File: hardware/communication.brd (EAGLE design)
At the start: 33.5 x 34.6 mm, 39 parts, among them J1 MICRO_USB_B_HIROSE_ZX62-B-5PA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, U2 NJM12888F, X1 FA-238

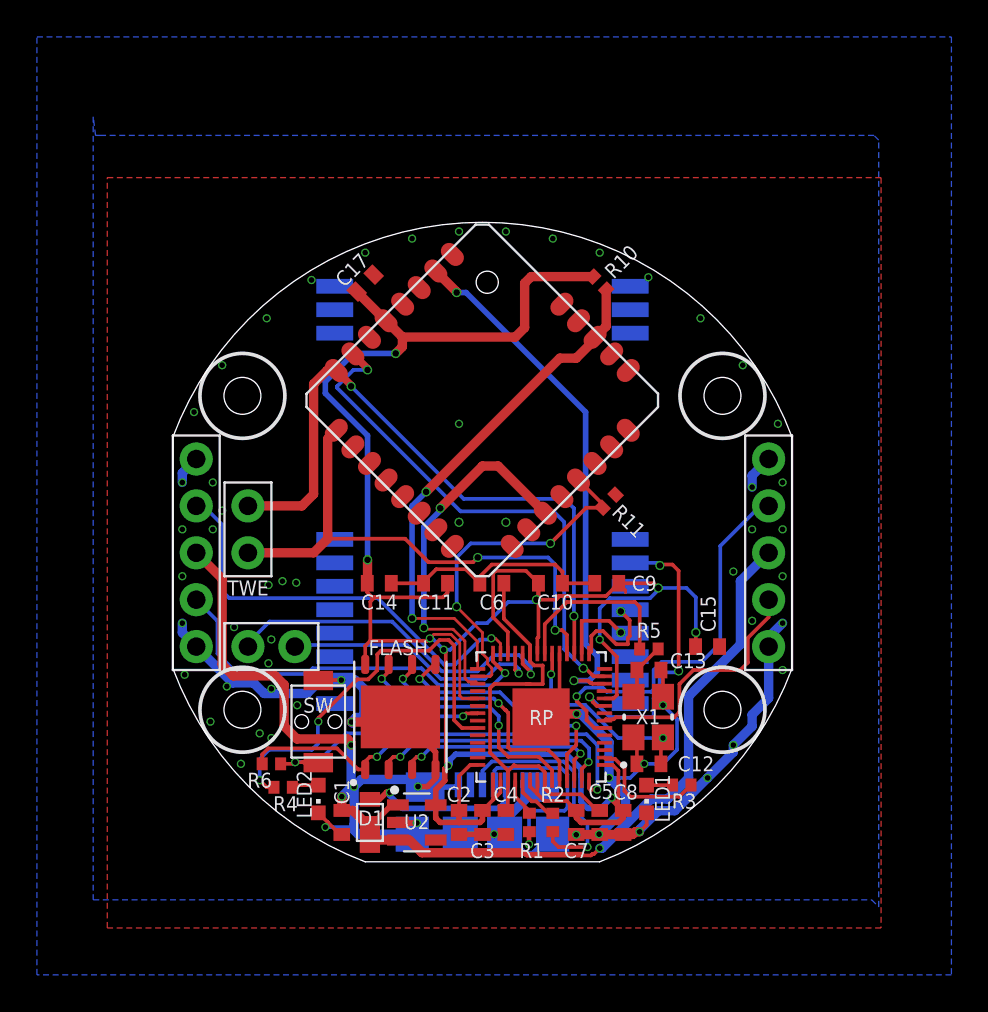
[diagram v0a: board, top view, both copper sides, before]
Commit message: communication_修正
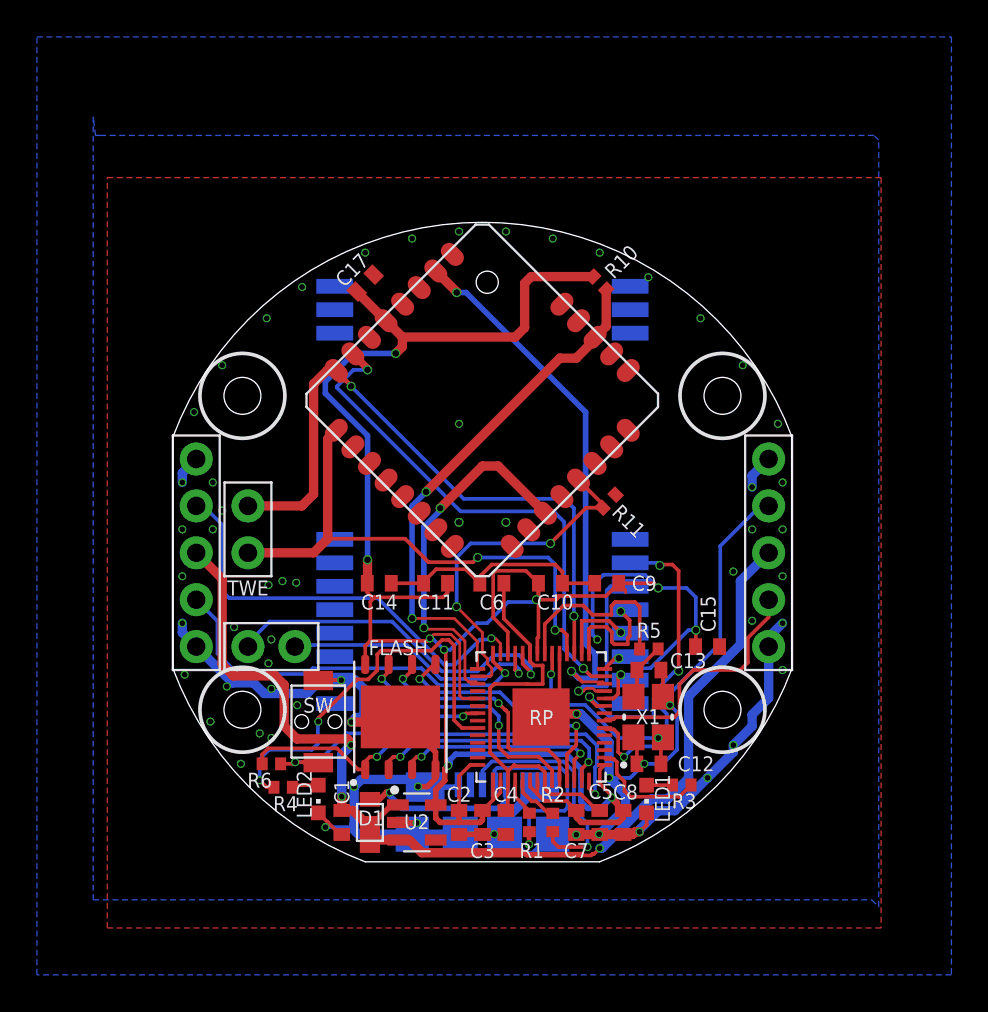
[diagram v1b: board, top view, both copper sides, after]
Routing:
- net LORA_M1: track 0.00 -> 9.72 mm, vias 0 -> 1
- net VDD: track 137.3 -> 142.1 mm, vias 10 -> 11
- net LORA_AUX: track 0.00 -> 1.67 mm, vias 0 -> 1
- net LORA_TRX: track 5.39 -> 6.74 mm
- net TWE_RTX: track 35.8 -> 36.5 mm
- net TX1: track 21.2 -> 20.5 mm
- net XOUT1: track 9.62 -> 10.3 mm
- net TWE_PGM: track 28.8 -> 29.4 mm
- net LORA_RTX: track 4.15 -> 4.67 mm

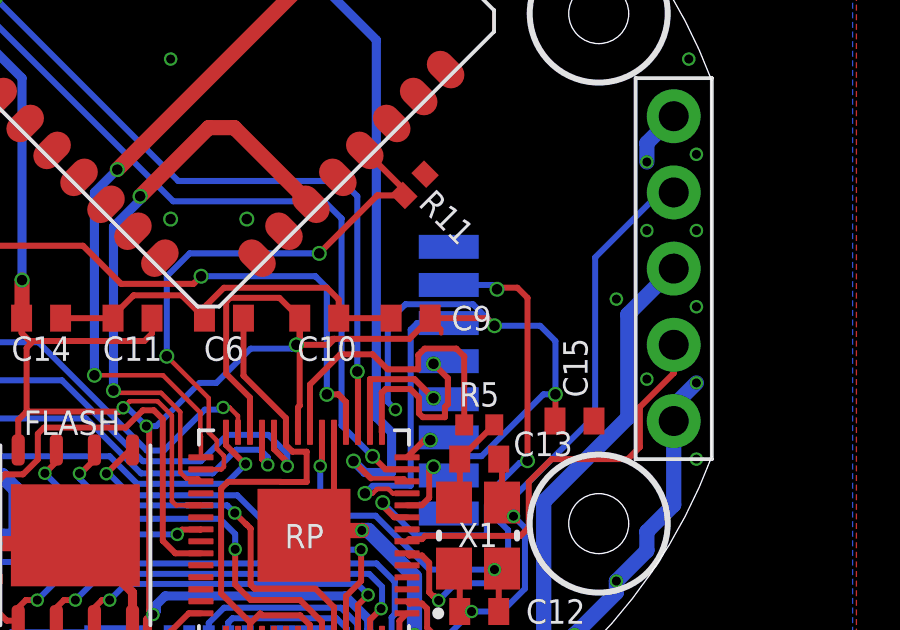
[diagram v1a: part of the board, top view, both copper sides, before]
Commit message: 回路微修正
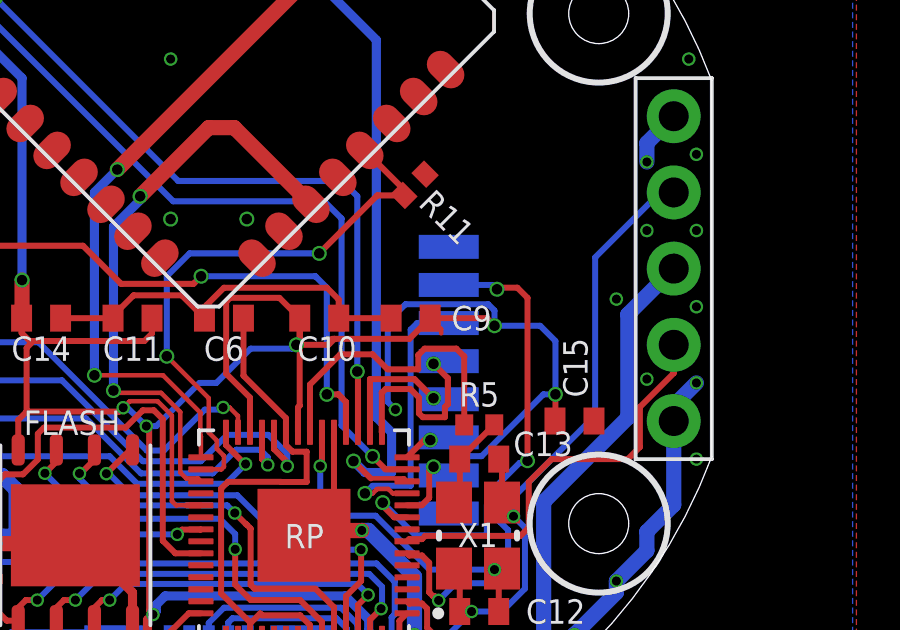
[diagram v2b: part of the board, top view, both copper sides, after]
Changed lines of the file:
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@@
 <param name="mdViaVia" value="5mil"/>
 <param name="mdSmdPad" value="5mil"/>
-<param name="mdSmdVia" value="5mil"/>
+<param name="mdSmdVia" value="0mil"/>
 <param name="mdSmdSmd" value="5mil"/>
 <param name="mdViaViaSameLayer" value="6mil"/>
@@
 <wire x1="9.271" y1="-1.651" x2="9.525" y2="-1.905" width="0.2" layer="1"/>
 <via x="9.525" y="-1.905" extent="1-16" drill="0.35"/>
-<wire x1="9.525" y1="-1.905" x2="8.807" y2="-1.187" width="0.2" layer="16"/>
-<wire x1="8.807" y1="-1.187" x2="6.56" y2="-1.187" width="0.2" layer="16"/>
+<wire x1="9.525" y1="-1.905" x2="9.525" y2="-1.397" width="0.2" layer="16"/>
+<wire x1="9.525" y1="-1.397" x2="9.315" y2="-1.187" width="0.2" layer="16"/>
+<wire x1="9.315" y1="-1.187" x2="6.56" y2="-1.187" width="0.2" layer="16"/>
 <wire x1="6.56" y1="-1.187" x2="5.969" y2="-1.778" width="0.2" layer="16"/>
 <wire x1="7.381" y1="-1.651" x2="6.692" y2="-2.34" width="0.2" layer="1"/>
